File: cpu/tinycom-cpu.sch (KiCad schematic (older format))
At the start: 10 parts, among them P1 CONN_02X08, P2 CONN_02X08, U1 OLIMEX_IC_A13, U2 H5TQG63BFR/FBGA96, Y1 Crystal

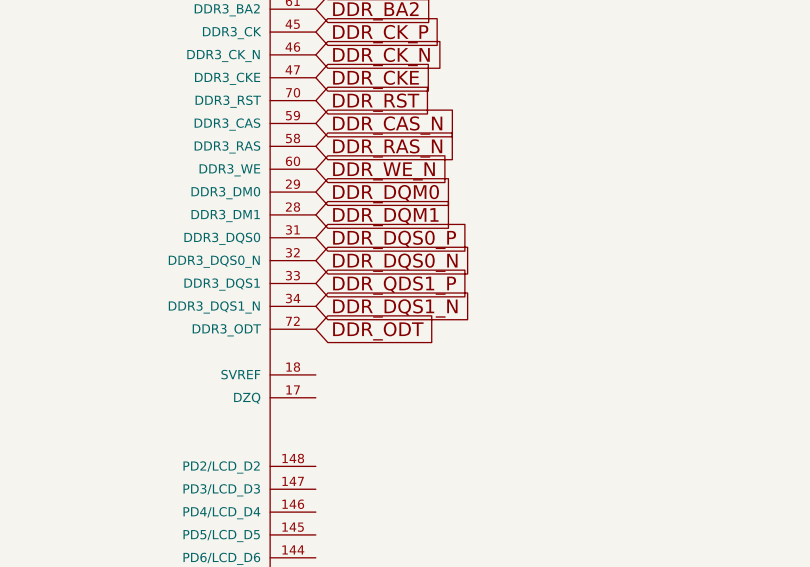
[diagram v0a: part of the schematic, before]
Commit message: fix ddr routing
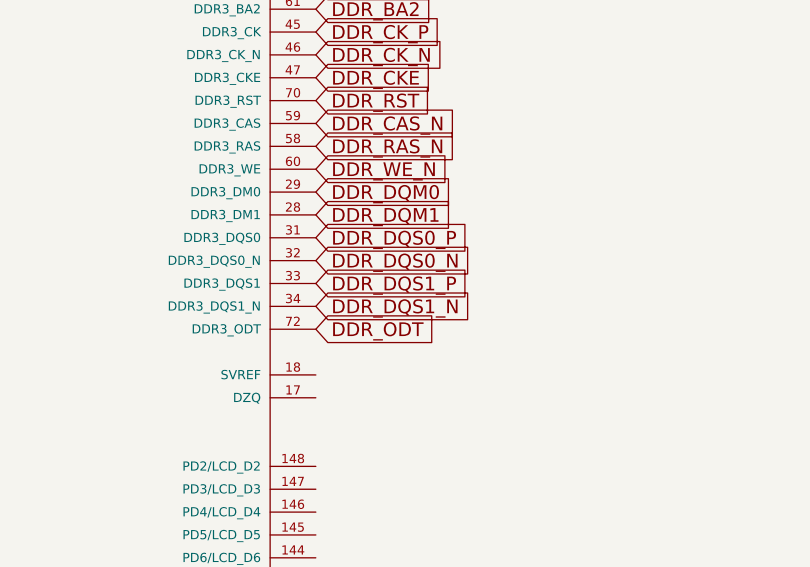
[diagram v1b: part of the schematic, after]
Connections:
- net DDR_QDS1_P is gone; now on net DDR_DQS1_P: U1.33 (DDR3_DQS1)
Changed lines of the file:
@@
 DDR_DQS0_N
 Text GLabel 5050 3200 2    60   Input ~ 0
-DDR_QDS1_P
+DDR_DQS1_P
 Text GLabel 5050 3300 2    60   Input ~ 0
 DDR_DQS1_N
@@
 MICIN1
 $Comp
-L GND #PWR?
+L GND #PWR015
 U 1 1 56250BEE
 P 11000 150
-F 0 "#PWR?" H 11000 -100 50  0001 C CNN
+F 0 "#PWR015" H 11000 -100 50  0001 C CNN
 F 1 "GND" H 11000 0   50  0000 C CNN
 F 2 "" H 11000 150 60  0000 C CNN
